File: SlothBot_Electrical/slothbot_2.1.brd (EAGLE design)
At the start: 121.9 x 72.1 mm, 25 parts

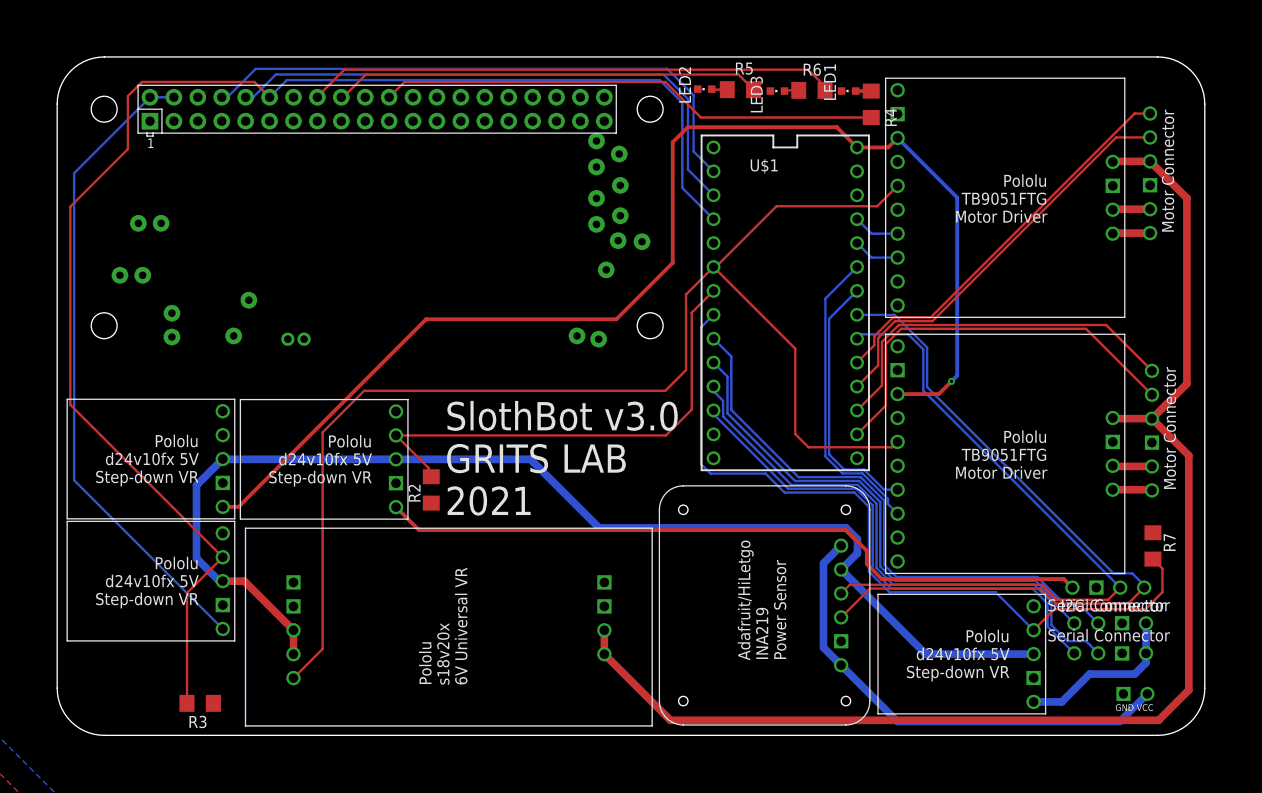
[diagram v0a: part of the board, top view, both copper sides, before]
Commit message: new pcb added
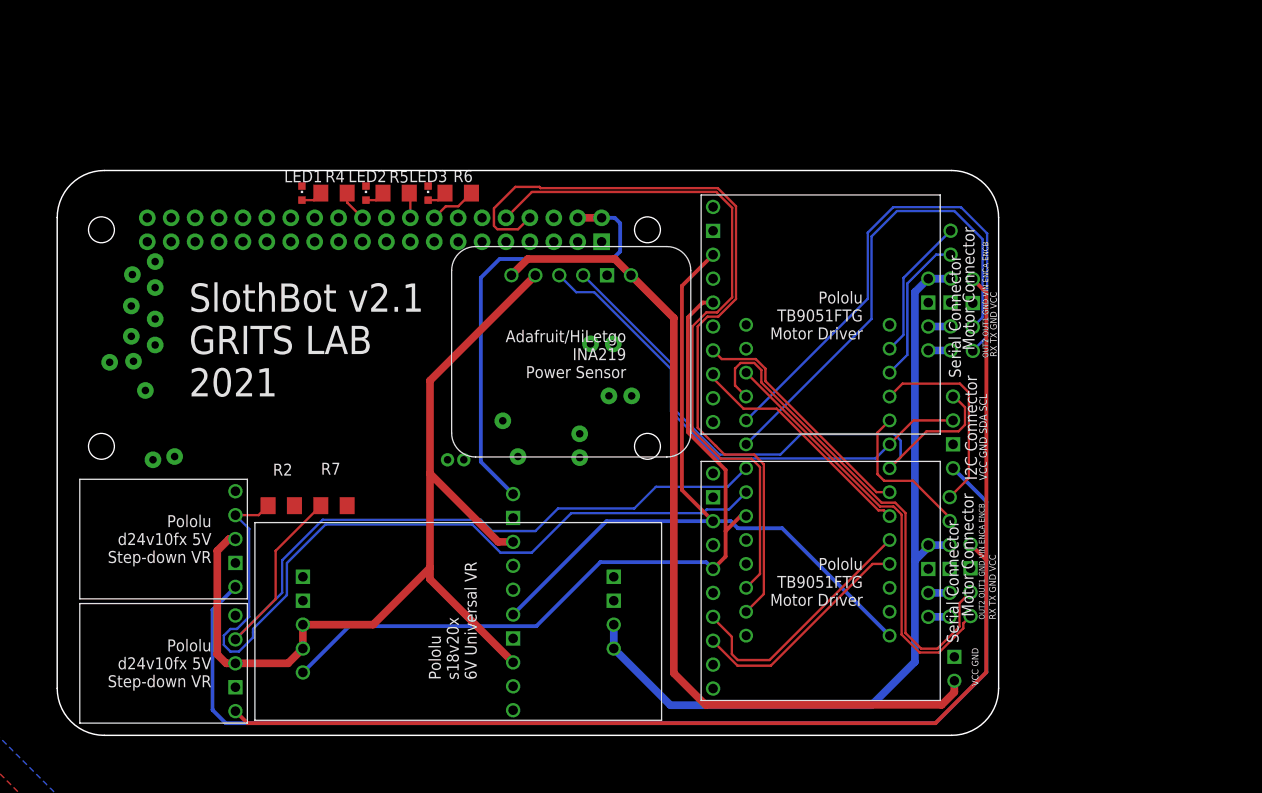
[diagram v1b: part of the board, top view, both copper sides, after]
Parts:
- removed R3: 10KΩ, adafruit:R3216
- moved R7 87.1 mm to (29.4, 24.4), turned to 180 degrees
- moved U$3 84.8 mm to (20.2, 14.0)
- moved U$2 66.0 mm to (66.2, 27.2), flipped to the bottom
- moved LED1 59.1 mm to (26.0, 57.6), turned to 0 degrees
- moved R4 57.8 mm to (29.4, 57.6), turned to 0 degrees
- moved U$12 46.1 mm to (49.7, 1.40), flipped to the bottom, turned to 0 degrees
- moved U$5 46.0 mm to (94.8, 12.6)
- moved U$10 45.2 mm to (93.8, 29.1)
- moved U$7 40.9 mm to (97.3, 48.5), turned to 270 degrees
- moved R6 39.1 mm to (42.6, 57.6)
- moved LED3 38.7 mm to (39.4, 57.6), turned to 0 degrees
- moved R5 38.2 mm to (36.0, 57.6)
- moved LED2 37.6 mm to (32.8, 57.6), turned to 0 degrees
- moved U$13 32.0 mm to (49.7, 14.2), flipped to the bottom, turned to 0 degrees
- moved U$4 26.1 mm to (94.9, 40.9)
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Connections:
- removed net RPI_EN: R3.2, U$1.2, U$13.SHDN, U$2.12
- net BACK_MOTOR_PWM1: now also U$1.23/A9; no longer U$1.22/A8
- net BACK_MOTOR_PWM2: now also U$1.22/A8; no longer U$1.23/A9
- net ENC_BACK_A: now also U$1.17/A3; no longer U$1.16/A2
- net ENC_BACK_B: now also U$1.16/A2; no longer U$1.17/A3
- net ENC_FRONT_A: now also U$1.15/A1; no longer U$1.14/A0
- net ENC_FRONT_B: now also U$1.14/A0; no longer U$1.15/A1
- net GND: no longer R3.1
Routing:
- net RPI_EN: track 151.0 -> 0.00 mm
- net N$2: track 17.9 -> 127.3 mm
- net MOTOR_EN: track 137.0 -> 83.8 mm
- net TEENSY_5V: track 132.2 -> 80.2 mm, vias 1 -> 0
- net N$12: track 56.3 -> 5.04 mm
- net 6V_MOTOR: track 138.0 -> 87.1 mm
- net N$14: track 53.4 -> 3.31 mm
- net N$9: track 76.2 -> 122.2 mm
- net N$13: track 45.5 -> 2.68 mm
- net 6V_BATT: track 50.5 -> 91.3 mm
- net I2C_SENSOR_EN: track 52.0 -> 87.6 mm
- net ENC_BACK_A: track 43.8 -> 16.2 mm
- net ENC_FRONT_A: track 42.7 -> 16.1 mm
- net ENC_FRONT_B: track 39.8 -> 15.2 mm
- net 6V_MONITORED: track 126.8 -> 103.4 mm
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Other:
- board size 121.9 x 72.1 mm -> 100 x 60 mm
- board text added: "OUT2 OUT1 GND VIN ENCA ENCB"
- board text added: "RX TX GND VCC"
- board text added: "SlothBot v2.1 GRITS LAB 2021"
- board text added: "VCC GND"
- board text added: "VCC GND SDA SCL"
- board text removed: "GND VCC"
- board text removed: "SlothBot v3.0 GRITS LAB 2021"
